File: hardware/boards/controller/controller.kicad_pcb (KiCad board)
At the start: 2 copper layers, 187 x 104.5 mm, 79 parts, among them J1 01x02, J10 01x05, J11 01x03, J2 01x06, J3 01x06, J4 01x02, J6 SMA, J7 02x04, J8 01x03, J9 01x05, SW1 Reset, SW2 Power, SW3 SW_SPDT, SW4 SW, SW5 SW, U1 ATmega328P, U10 Joystick, U2 AMS1117-5.0, U3 AMS1117-3.3, U4 ILI9341, U7 NRF24L01, U8 RFX2401C, U9 Joystick, Y1 16MHz, Y3 16MHz

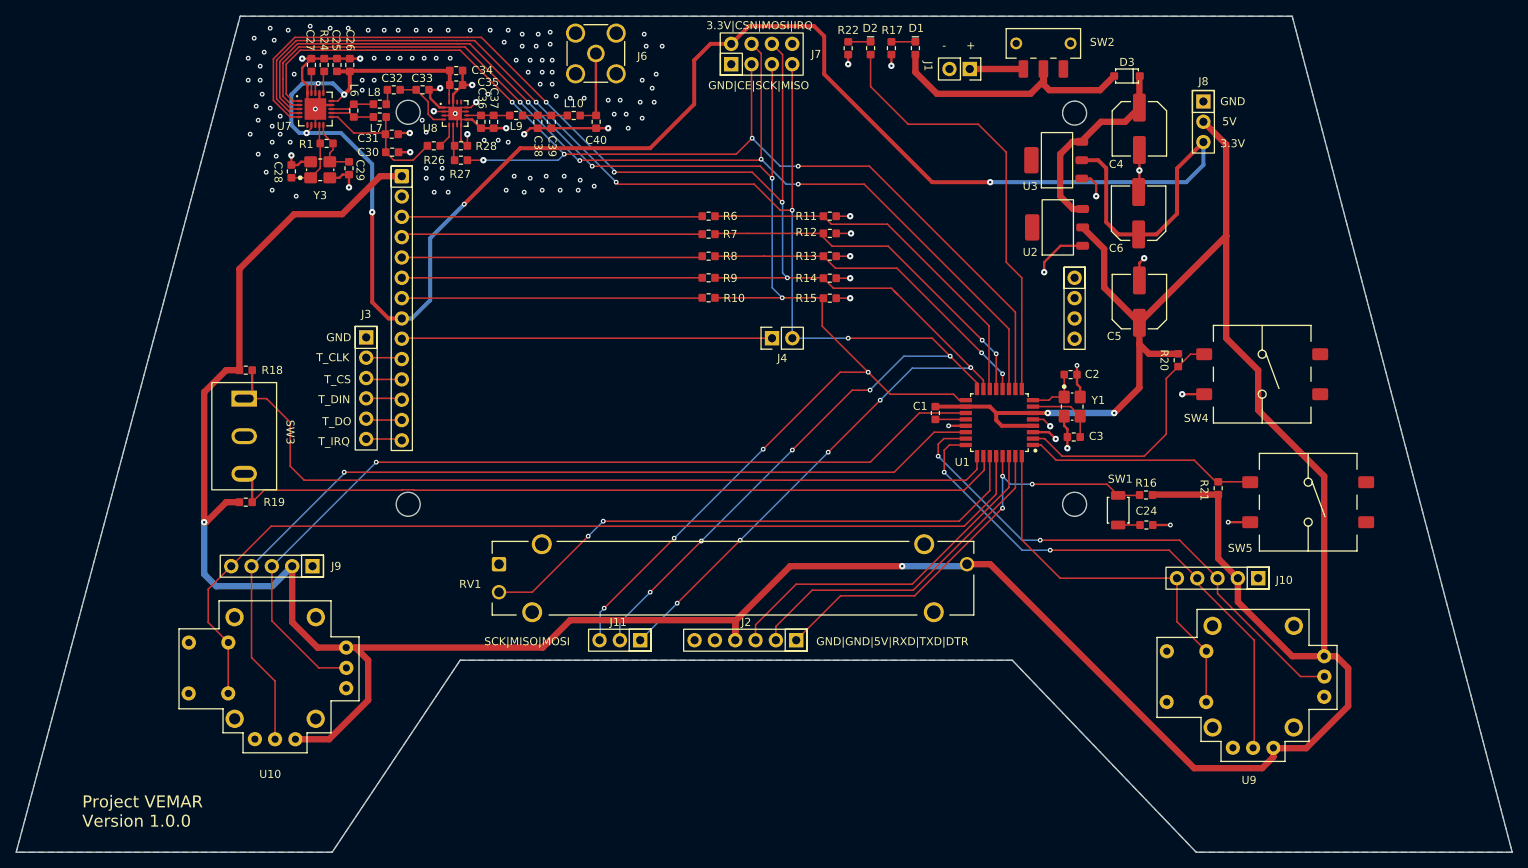
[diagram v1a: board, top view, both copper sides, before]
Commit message: new version for pcb controller
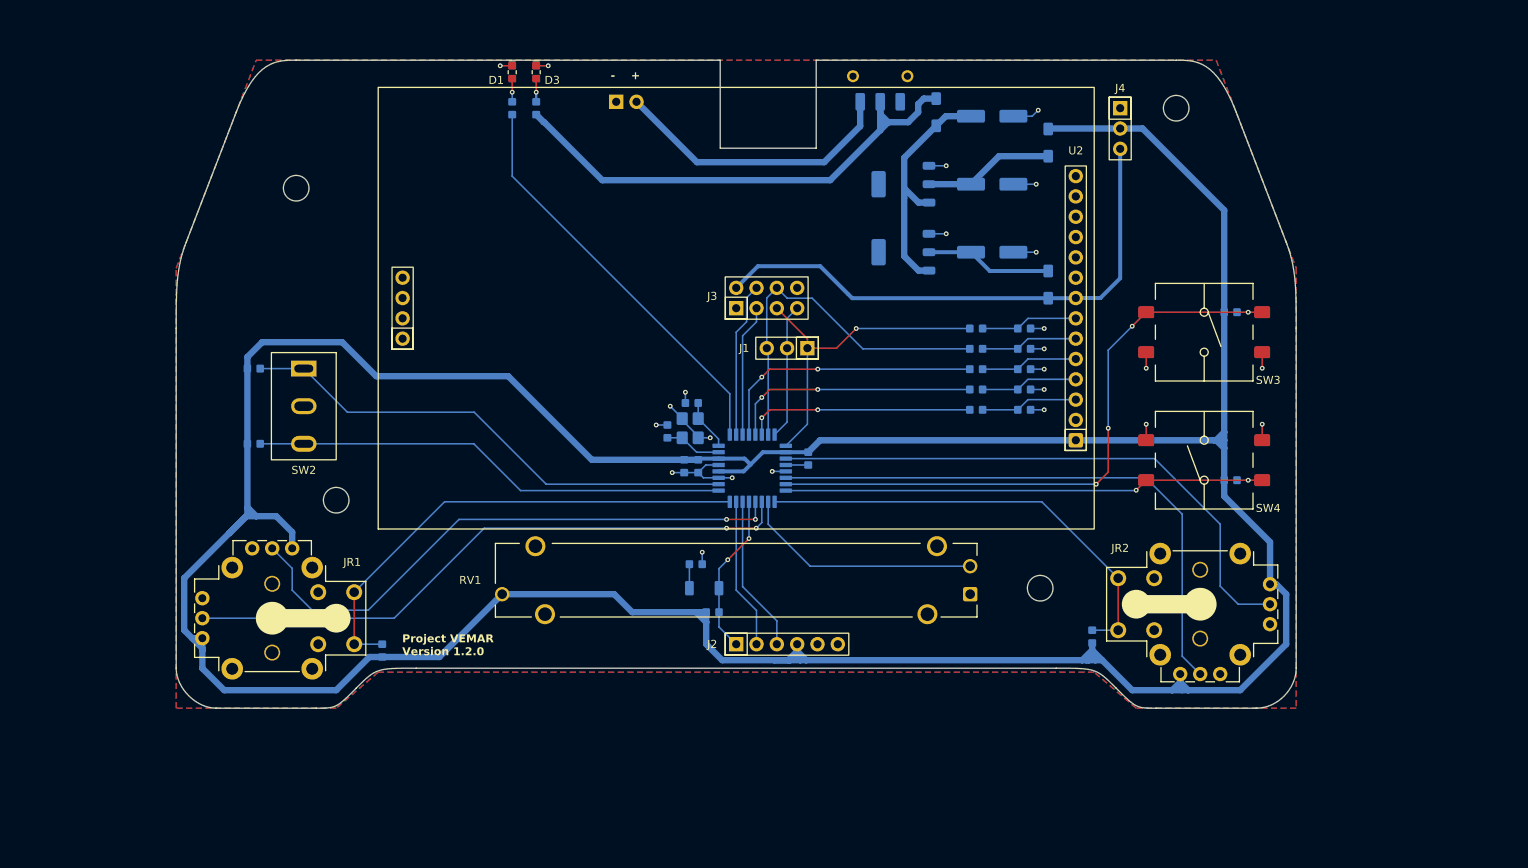
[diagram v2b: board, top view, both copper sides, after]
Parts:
- removed C24: 100nF, common:C_0603
- removed C25: 10nF, common:C_0603
- removed C26: 1nF, common:C_0603
- removed C27: 33nF, common:C_0603
- removed C28, C29: 22pF, common:C_0603
- removed C30: 2.2nF, common:C_0603
- removed C31: 4.7nF, common:C_0603
- removed C32, C37, C38, C39, C40: 1.5pF, common:C_0603
- removed C33: 1.0pF, common:C_0603
- removed C34: 220pF, common:C_0603
- removed C35: 1uF, common:C_0603
- removed C36: 0.3pF, common:C_0603
- removed J10, J9: 01x05, connector:Pin_01x05
- removed J11, J8: 01x03, connector:Pin_01x03
- removed J6: SMA, connector:SMA
- removed J7: 02x04, connector:Pin_02x04
- removed L10, L9: 2.4nH, common:L_0603
- removed L6: 8.2nH, common:L_0603
- removed L7: 2.7nH, common:L_0603
- removed L8: 3.9nH, common:L_0603
- removed R20, R21: 10k, common:R_0603
- removed R22: 330, common:R_0603
- removed R24: 22k, common:R_0603
- removed R26, R27: 1k, common:R_0603
- removed R28: 20k, common:R_0603
- removed U10, U9: Joystick, misc:Joystick
- removed U7: NRF24L01, transceiver:NRF24L01_QFN20
- removed U8: RFX2401C, transceiver:RFX2401C_QFN16
- removed Y3: 16MHz, common:Crystal_3225
- added C7: 22uF, common:C_D6.3xL5.4, B.Cu at (182.0, 64.5)
- added C8: 22uF, common:C_D6.3xL5.4, B.Cu at (182.0, 73.0)
- added C9: 100uF, common:C_D6.3xL5.4, B.Cu at (182.0, 56.0)
- added D4: Diode, common:D_SOD123FL, B.Cu at (189.0, 59.3)
- added D5: Diode, common:D_SOD123FL, B.Cu at (189.0, 77.0)
- added J5: 01x02, connector:Pin_01x02, B.Cu at (135.0, 54.2)
- added JR1: Joystick, misc:Joystick, F.Cu at (92.0, 118.8)
- added JR2: Joystick, misc:Joystick, F.Cu at (208.0, 117.0)
- added R2: 10k, common:R_0603, B.Cu at (89.7, 97.0)
- added R3: 10k, common:R_0603, B.Cu at (89.7, 87.5)
- added R4: 10k, common:R_0603, B.Cu at (211.8, 101.5)
- added R5: 10k, common:R_0603, B.Cu at (211.8, 80.5)
- added REF**: MountingHole_3.2mm_M3, connector:MountingHole_3.2mm_M3, F.Cu at (188.0, 115.0)
- added REF**: MountingHole_3.2mm_M3, connector:MountingHole_3.2mm_M3, F.Cu at (205.0, 55.0)
- added REF**: MountingHole_3.2mm_M3, connector:MountingHole_3.2mm_M3, F.Cu at (100.0, 104.0)
- added REF**: MountingHole_3.2mm_M3, connector:MountingHole_3.2mm_M3, F.Cu at (95.0, 65.0)
- C1: value 100nF -> 1uF; moved to B.Cu
- C2, C3: value 22pF -> 100nF; moved to B.Cu
- C4: value 100uF -> 100nF; footprint common:C_D6.3xL5.4 -> common:C_0603; moved to B.Cu
- C5, C6: value 22uF -> 12pF; footprint common:C_D6.3xL5.4 -> common:C_0603; moved to B.Cu
- D1: value Red -> Green
- D2: value ~ -> Diode; footprint common:LED_0603 -> common:D_SOD123FL; moved to B.Cu
- D3: value Diode -> Red; footprint common:D_SOD123 -> common:LED_0603
- J1, J4: value 01x02 -> 01x03; footprint connector:Pin_01x02 -> connector:Pin_01x03
- J3: value 01x06 -> 02x04; footprint connector:Pin_01x06 -> connector:Pin_02x04
- R1: value 1M -> 10k; moved to B.Cu
- R10, R14, R15, R9, SW1, U1, Y1: moved to B.Cu
- R11, R12, R13: value 2k -> 1k; moved to B.Cu
- R16, R18: value 10k -> 2k; moved to B.Cu
- R17: value 1k -> 2k; moved to B.Cu
- R19: value 10k -> 1k; moved to B.Cu
- R6: value 1k -> 330; moved to B.Cu
- R7, R8: value 1k -> 10k; moved to B.Cu
- SW2: value Power -> SW_SPDT; footprint switch:SW_Slide9.1x3.5 -> common:SW_Toggle
- SW3: value SW_SPDT -> SW; footprint common:SW_Toggle -> switch:SW_Tactile12x12
- SW5: value SW -> Power; footprint switch:SW_Tactile12x12 -> switch:SW_Slide9.1x3.5; moved to B.Cu
- U2: value AMS1117-5.0 -> ILI9341; footprint regulator:AMS1117-SOT223 -> display:ILI9341
- U3: value AMS1117-3.3 -> AMS1117-5.0; moved to B.Cu
- U4: value ILI9341 -> AMS1117-3.3; footprint display:ILI9341 -> regulator:AMS1117-SOT223; moved to B.Cu
- moved SW3 120.7 mm to (208.5, 83.0), turned to 0 degrees
- moved SW2 103.0 mm to (96.0, 92.2), turned to -90 degrees
- moved R18 97.4 mm to (186.0, 92.7)
- moved R1 75.9 mm to (147.1, 118.0), turned to 180 degrees
- moved SW5 75.5 mm to (168.0, 51.0), turned to 180 degrees
- moved D3 73.9 mm to (125.0, 50.5), turned to -90 degrees
- moved R8 67.5 mm to (194.5, 121.0), turned to -90 degrees
- moved R7 66.1 mm to (105.8, 122.8), turned to 90 degrees
- moved C6 64.9 mm to (141.4, 95.4), turned to -90 degrees
- moved R19 61.2 mm to (125.0, 55.0), turned to -90 degrees
- moved C4 58.4 mm to (159.0, 98.8)
- moved C5 57.4 mm to (144.4, 91.8), turned to 0 degrees
- moved SW1 52.7 mm to (146.0, 115.0), turned to 0 degrees
- moved J4 52.2 mm to (198.0, 55.0), turned to 0 degrees
- moved D1 50.5 mm to (122.0, 50.5)
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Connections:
- C1 pad 1: +5V -> GND
- C1 pad 2: Net-(U1-AREF) -> +5V
- C2 pad 2: Net-(U1-PCINT7/XTAL2/TOSC2/PB7) -> +5V
- C3 pad 2: Net-(U1-PCINT6/XTAL1/TOSC1/PB6) -> Net-(C3-Pad2)
- C4 pad 1: +BATTERY -> +5V
- C4 pad 2: GND -> Net-(U1-AREF)
- C5 pad 1: +5V -> GND
- C5 pad 2: GND -> Net-(U1-PCINT7/XTAL2/TOSC2/PB7)
- C6 pad 1: +3.3V -> GND
- C6 pad 2: GND -> Net-(U1-PCINT6/XTAL1/TOSC1/PB6)
- D1 pad 1: Net-(D1-K) -> GND
- D2 pad 1: Net-(D2-K) -> +BATTERY
- D3 pad 1: +BATTERY -> GND
- D3 pad 2: Net-(D1-A) -> Net-(D3-A)
- J1 pad 1: Net-(J1-Pad1) -> SCK
- J1 pad 2: GND -> MISO
- J3 pad 2: Net-(U4-T_CLK) -> CE
- J3 pad 3: Net-(U4-T_CS) -> SCK
- J3 pad 4: Net-(U4-T_DIN) -> MISO
- J3 pad 5: Net-(U4-T_DO) -> unconnected-(J3-Pad5)
- J3 pad 6: Net-(U4-T_IRQ) -> MOSI
- J4 pad 1: Net-(U4-MISO) -> GND
- J4 pad 2: MISO -> +5V
- R1 pad 1: Net-(U7-XC2) -> DTR
- R1 pad 2: Net-(U7-XC1) -> +5V
- R10 pad 1: SCK -> Net-(U2-MOSI)
- R10 pad 2: Net-(U4-SCK) -> MOSI
- R11 pad 1: GND -> Net-(U2-D/~{C})
- R11 pad 2: CS -> DC
- R12 pad 1: GND -> Net-(U2-RESET)
- R13 pad 1: GND -> Net-(U2-~{CS})
- R13 pad 2: DC -> CS
- R14 pad 2: MOSI -> Net-(U2-SCK)
- R15 pad 2: SCK -> Net-(U2-MOSI)
- R16 pad 1: DTR -> GND
- R16 pad 2: +5V -> Net-(U2-D/~{C})
- R17 pad 2: Net-(D1-K) -> Net-(U2-RESET)
- R18 pad 1: Net-(U1-PC2/ADC2/PCINT10) -> GND
- R18 pad 2: +5V -> Net-(U2-~{CS})
- R19 pad 1: Net-(U1-PC3/ADC3/PCINT11) -> Net-(D3-A)
- R19 pad 2: +5V -> Net-(D2-A)
- R6 pad 1: CS -> Net-(D1-A)
- R6 pad 2: Net-(U4-~{CS}) -> LED
- R7 pad 1: RESET -> +5V
- R7 pad 2: Net-(U4-RESET) -> JOY1-B
- R8 pad 1: DC -> JOY2-B
- R8 pad 2: Net-(U4-D/~{C}) -> +5V
- R9 pad 1: MOSI -> Net-(U2-SCK)
- R9 pad 2: Net-(U4-MOSI) -> SCK
- RV1 pad 2: Net-(U1-PC4/ADC4/SDA/PCINT12) -> Net-(U1-PC3/ADC3/PCINT11)
- RV1 pad 4: (no net) -> unconnected-(RV1-DNC-Pad4)
- RV1 pad 5: (no net) -> unconnected-(RV1-DNC-Pad5)
- RV1 pad 6: (no net) -> unconnected-(RV1-DNC-Pad6)
- RV1 pad 7: (no net) -> unconnected-(RV1-DNC-Pad7)
- SW1 pad 1: Net-(C24-Pad2) -> Net-(C3-Pad2)
- SW2 pad 1: Net-(J1-Pad1) -> TOGGLE2
- SW2 pad 2: Net-(D1-A) -> GND
- SW2 pad 3: (no net) -> TOGGLE1
- SW3 pad 1: Net-(U1-PC2/ADC2/PCINT10) -> BTN1
- SW3 pad 2: GND -> BTN1
- SW3 pad 3: Net-(U1-PC3/ADC3/PCINT11) -> GND
- SW4 pad 1: Net-(U1-PCINT20/XCK/T0/PD4) -> BTN2
- SW4 pad 2: unconnected-(SW4-Pad2) -> BTN2
- SW4 pad 4: unconnected-(SW4-Pad4) -> GND
- SW5 pad 1: Net-(U1-PCINT19/OC2B/INT1/PD3) -> unconnected-(SW5-Pad1)
- SW5 pad 2: unconnected-(SW5-Pad2) -> Net-(D2-A)
- SW5 pad 3: GND -> Net-(J5-Pad2)
- U1 pad 1: Net-(U1-PCINT19/OC2B/INT1/PD3) -> TOGGLE1
- U1 pad 10: CE -> CSN
- U1 pad 11: CSN -> CE
- U1 pad 19: Net-(U1-ADC6) -> JOY2-Y
- U1 pad 2: Net-(U1-PCINT20/XCK/T0/PD4) -> TOGGLE2
- U1 pad 22: Net-(U1-ADC7) -> JOY2-X
- U1 pad 23: JOY1-X -> BTN1
- U1 pad 24: JOY1-Y -> BTN2
- U1 pad 25: Net-(U1-PC2/ADC2/PCINT10) -> JOY2-B
- U1 pad 27: Net-(U1-PC4/ADC4/SDA/PCINT12) -> JOY1-X
- U1 pad 28: Net-(U1-PC5/ADC5/SCL/PCINT13) -> JOY1-Y
- U1 pad 9: Net-(D2-A) -> LED
- U2 pad 1: GND -> +5V
- U2 pad 2: +5V -> GND
- U2 pad 3: +BATTERY -> Net-(U2-~{CS})
- U2 pad 4: (no net) -> Net-(U2-RESET)
- U3 pad 2: +3.3V -> Net-(D4-A)
- U3 pad 4: (no net) -> unconnected-(U3-DNC-Pad4)
- U4 pad 1: +5V -> GND
- U4 pad 2: GND -> Net-(D5-A)
- U4 pad 3: Net-(U4-~{CS}) -> +BATTERY
- U4 pad 4: Net-(U4-RESET) -> unconnected-(U4-DNC-Pad4)
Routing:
- net MISO: track 199.6 -> 17.0 mm, vias 9 -> 0
- net +3.3V: track 239.8 -> 68.0 mm, vias 6 -> 0
- net MOSI: track 208.4 -> 46.2 mm, vias 9 -> 0
- net SCK: track 194.8 -> 41.2 mm, vias 8 -> 1
- net CE: track 144.1 -> 16.5 mm, vias 5 -> 0
- net Net-(U1-PC5/ADC5/SCL/PCINT13): track 122.2 -> 0.00 mm
- net Net-(U1-ADC7): track 119.2 -> 0.00 mm, vias 1 -> 0
- net CSN: track 135.5 -> 19.4 mm, vias 4 -> 0
- net Net-(U1-ADC6): track 113.2 -> 0.00 mm, vias 1 -> 0
- net Net-(U1-PC2/ADC2/PCINT10): track 105.2 -> 0.00 mm
- net BTN1: track 0.00 -> 78.8 mm, vias 0 -> 4
- net GND: track 132.0 -> 56.7 mm, vias 138 -> 24
- net JOY2-Y: track 0.00 -> 72.6 mm
- net JOY2-X: track 0.00 -> 72.4 mm
- net Net-(U1-PC4/ADC4/SDA/PCINT12): track 70.9 -> 0.00 mm, vias 2 -> 0
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- added copper zone on F.Cu, net GND
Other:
- board size 187 x 104.5 mm -> 140 x 81 mm
- board text added: "3V3"
- board text added: "CE"
- board text added: "D/~{C}"
- board text added: "DTR"
- board text added: "MISO"
- board text added: "MOSI"
- board text added: "Project VEMAR Version 1.2.0"
- board text added: "RESET"
- board text added: "RXD"
- board text added: "SCK"
- board text added: "TXD"
- board text added: "VCC"
- board text added: "| 3V3"
- board text added: "| CSN"
- board text added: "| IRQ"
- board text added: "| MOSI"
- board text added: "~{CS}"
- board text removed: "3.3V"
- board text removed: "3.3V|CSN|MOSI|IRQ"
- board text removed: "GND|CE|SCK|MISO"
- board text removed: "GND|GND|5V|RXD|TXD|DTR"
- board text removed: "Project VEMAR Version 1.0.0"
- board text removed: "SCK|MISO|MOSI"
- board text removed: "T_CLK"
- board text removed: "T_CS"
- board text removed: "T_DIN"
- board text removed: "T_DO"
- board text removed: "T_IRQ"
